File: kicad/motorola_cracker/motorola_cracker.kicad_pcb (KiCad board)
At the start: 2 copper layers, 115.1 x 46.5 mm, 28 parts, among them J1 DB9, P1 CONN_6, P2 CONN_2, P3 CONN_6, SW1 SWITCH_INV, U1 78L10, U2 74LS245, U3 MAX232, U4 78L05, U5 68HC05_PLCC, X1 4Mhz

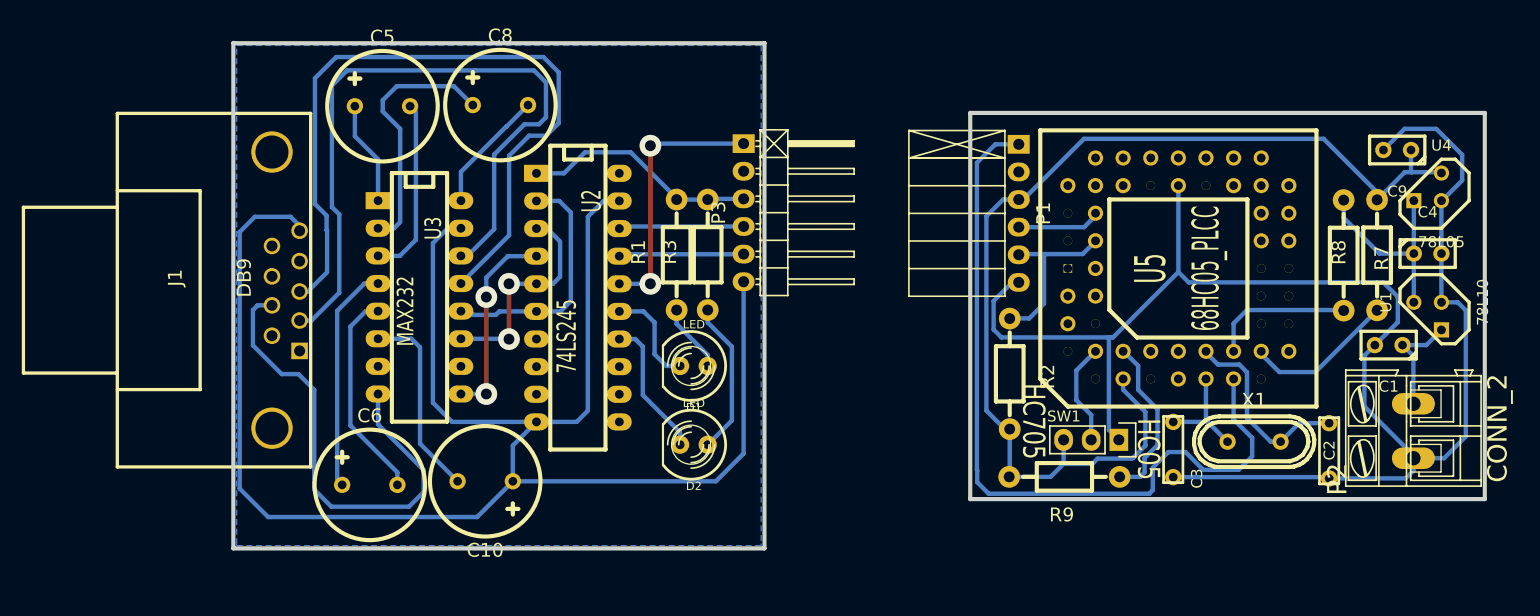
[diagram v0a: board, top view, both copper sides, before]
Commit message: motorola cracker simple board for usb to serial dongle (tested with cp2102)
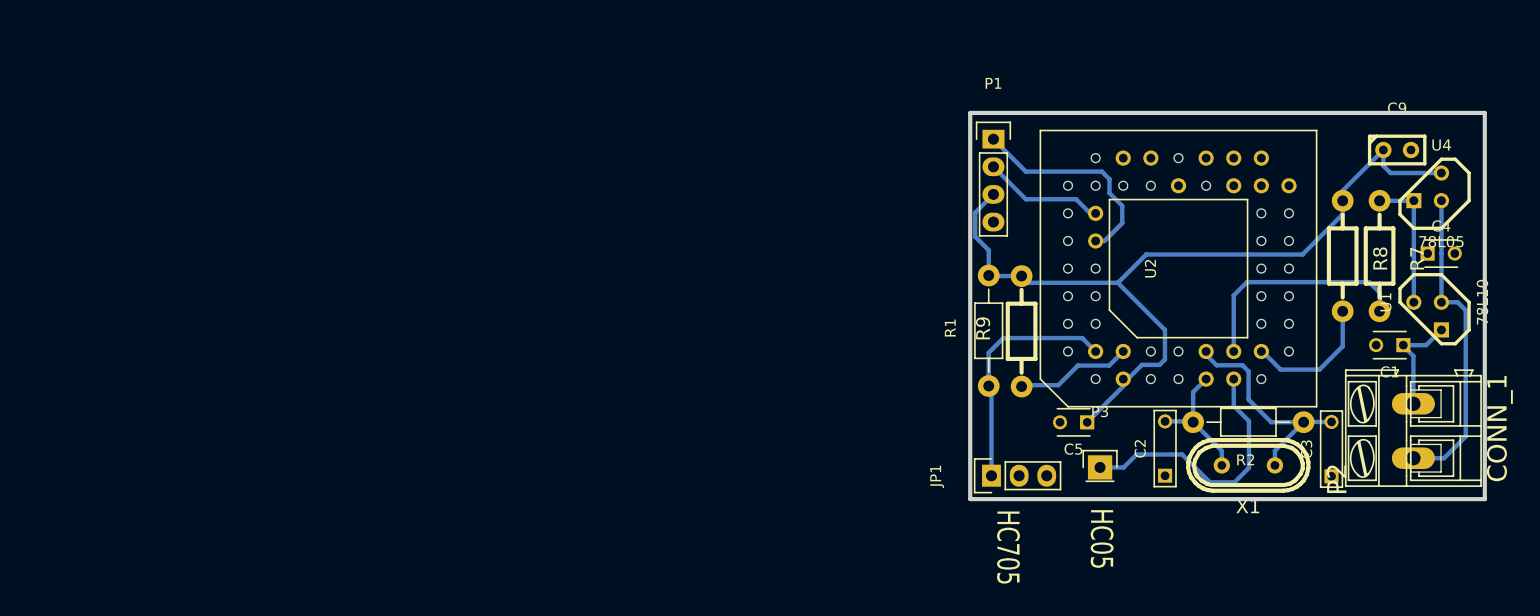
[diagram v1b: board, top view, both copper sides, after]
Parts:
- removed C10, C6, C8: 10m, Capacitors_Elko_ThroughHole:Elko_vert_DM10_RM5
- removed D1, D2: LED, LEDs:LED-5MM
- removed J1: DB9, Connect:DB9FC
- removed R3: 1k, Resistors_ThroughHole:Resistor_Horizontal_RM10mm
- removed SW1: SWITCH_INV, Pin_Headers:Pin_Header_Straight_1x03
- removed U3: MAX232, Sockets_DIP:DIP-16__300_ELL
- removed U5: 68HC05_PLCC, Sockets:PLCC52
- added JP1: JUMPER3, Pin_Headers:Pin_Header_Straight_1x03, F.Cu at (186.4, 117.9)
- C1, C4: footprint Capacitors_ThroughHole:Capacitor3MMDiscRM2.5 -> Capacitors_ThroughHole:C_Disc_D3_P2.5
- C2, C3: footprint Capacitors_ThroughHole:Capacitor6MMDiscRM5 -> Capacitors_ThroughHole:C_Rect_L7_W2_P5
- C5: value 10m -> 100n; footprint Capacitors_Elko_ThroughHole:Elko_vert_DM10_RM5 -> Capacitors_ThroughHole:C_Disc_D3_P2.5
- P1: value CONN_6 -> CONN_4; footprint Socket_Strips:Socket_Strip_Angled_1x06 -> Pin_Headers:Pin_Header_Straight_1x04
- P2: value CONN_2 -> CONN_1
- P3: value CONN_6 -> CONN_5; footprint Pin_Headers:Pin_Header_Angled_1x06 -> Pin_Headers:Pin_Header_Straight_1x01
- R1: value 1k -> 10k
- R2: value 4k7 -> 100M
- R8, R9: value 2k -> 1k
- U2: value 74LS245 -> 68HC05_PLCC; footprint Sockets_DIP:DIP-20__300_ELL -> Sockets:PLCC52
- moved C5 71.0 mm to (195.2, 112.9), turned to 180 degrees
- moved U2 55.3 mm to (203.6, 98.8), turned to 90 degrees
- moved P3 40.3 mm to (196.4, 117.1), turned to 0 degrees
- moved R1 29.5 mm to (186.2, 104.5)
- moved R2 22.4 mm to (210.1, 112.9), turned to 180 degrees
- moved C2 15.3 mm to (202.4, 117.9)
- moved C3 14.8 mm to (217.7, 117.9)
- moved R9 14.0 mm to (189.2, 104.6), turned to 90 degrees
- moved P1 7.21 mm to (186.6, 86.9), turned to 0 degrees
- moved R7 3.30 mm to (222.1, 97.7)
- moved R8 3.16 mm to (218.7, 97.7), turned to 270 degrees
- moved X1 2.24 mm to (210.1, 116.9), turned to 180 degrees
- moved C1 1.35 mm to (224.3, 105.8)
- turned C9 to 0 degrees
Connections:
- net +10V renamed /+10V
- C5 pad 1: Net-(C5-Pad1) -> +5V
- C5 pad 2: Net-(C5-Pad2) -> GND
- P1 pad 1: 68_18 -> /TX
- P1 pad 2: (no net) -> /RX
- P1 pad 4: 68_50 -> GND
- P3 pad 1: 68_18 -> /RESET
- R1 pad 1: Net-(D1-Pad1) -> Net-(JP1-Pad1)
- R2 pad 1: 68_52 -> Net-(C3-Pad2)
- R2 pad 2: +5V -> Net-(C2-Pad2)
- R8 pad 1: Net-(R8-Pad1) -> +5V
- R8 pad 2: +5V -> Net-(R8-Pad2)
- U2 pad 10: GND -> +5V
- U2 pad 11: (no net) -> Net-(R9-Pad1)
- U2 pad 14: Net-(D2-Pad2) -> (no net)
- U2 pad 15: Net-(D1-Pad2) -> (no net)
- U2 pad 16: 68_18 -> Net-(C2-Pad2)
- U2 pad 17: 68_52 -> Net-(C3-Pad2)
- U2 pad 18: 68_50 -> /RESET
- U2 pad 19: GND -> Net-(R7-Pad2)
- U2 pad 2: Rx -> (no net)
- U2 pad 3: Tx -> (no net)
- U2 pad 4: Reset -> (no net)
- U2 pad 5: Tx -> (no net)
- U2 pad 6: Rx -> (no net)
- U2 pad 9: (no net) -> Net-(JP1-Pad1)
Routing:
- net GND: track 306.8 -> 29.5 mm
- net 68_18: track 95.7 -> 0.00 mm, vias 2 -> 0
- net Net-(J1-Pad3): track 69.5 -> 0.00 mm
- net Net-(J1-Pad2): track 65.7 -> 0.00 mm
- net Net-(J1-Pad7): track 43.7 -> 0.00 mm
- net +5V: track 120.8 -> 78.1 mm
- net 68_52: track 27.7 -> 0.00 mm
- net /RESET: track 0.00 -> 24.5 mm
- net Net-(C8-Pad1): track 23.7 -> 0.00 mm
- net Rx: track 22.8 -> 0.00 mm
- net Net-(JP1-Pad1): track 0.00 -> 22.4 mm
- net Net-(C6-Pad1): track 21.8 -> 0.00 mm
- net Tx: track 20.5 -> 0.00 mm, vias 2 -> 0
- net Net-(C6-Pad2): track 20.4 -> 0.00 mm
- net /TX: track 0.00 -> 19.9 mm
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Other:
- board size 115.1 x 46.5 mm -> 47.3 x 35.5 mm

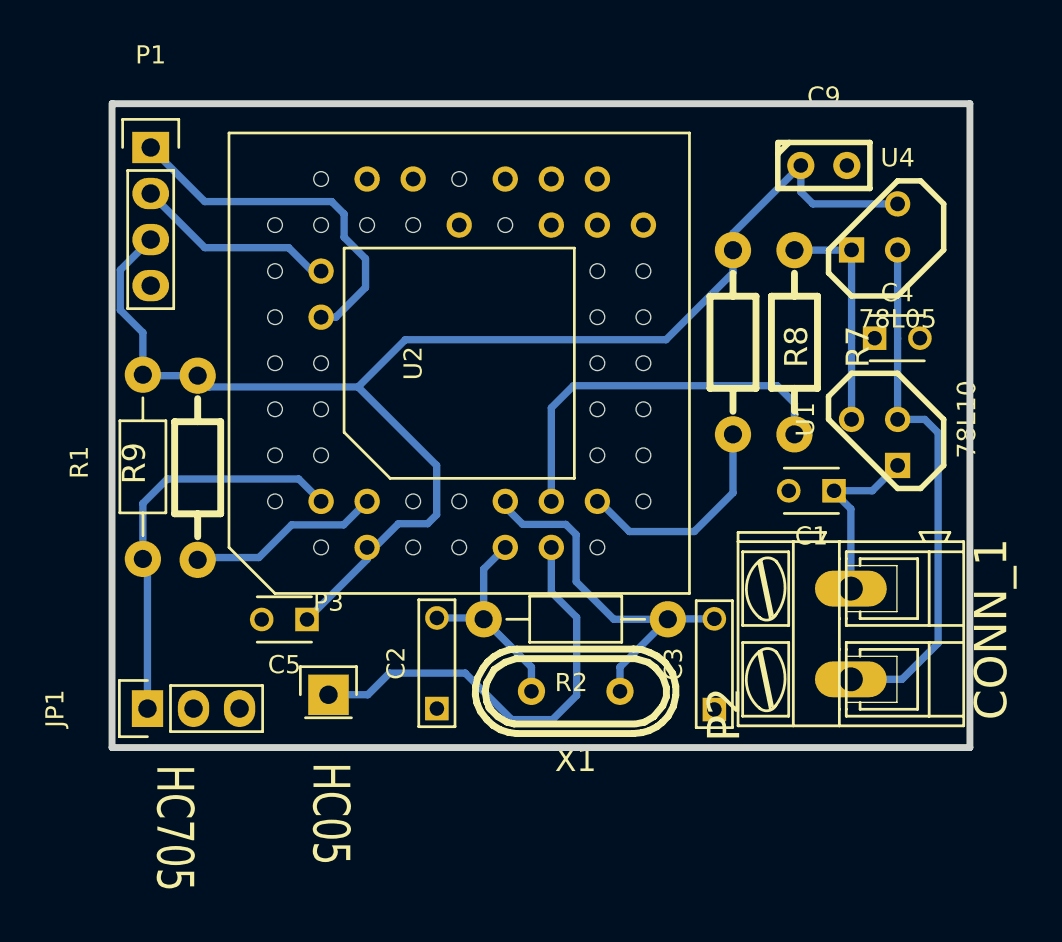
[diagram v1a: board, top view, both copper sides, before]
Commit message: simplified version
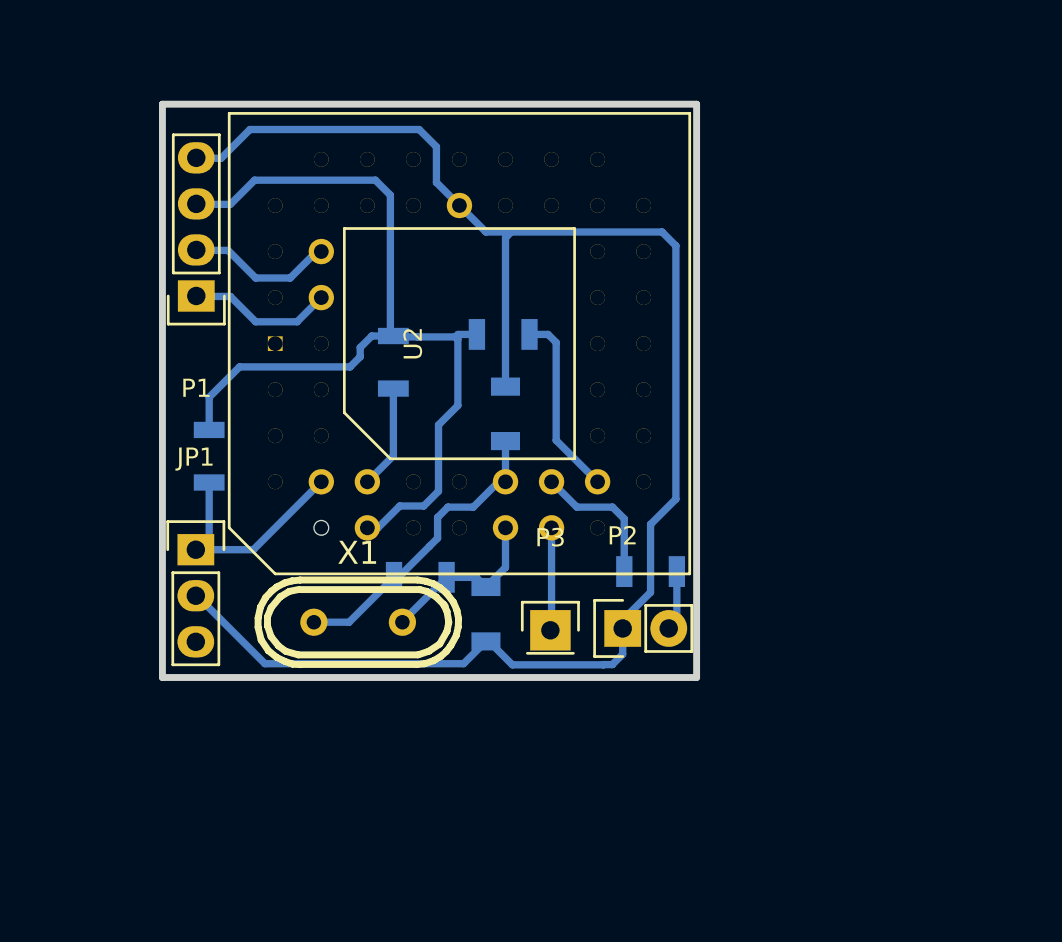
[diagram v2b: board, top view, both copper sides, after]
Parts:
- removed C1, C4, C5: 100n, Capacitors_ThroughHole:C_Disc_D3_P2.5
- removed C9: 100n, Capacitors_ThroughHole:Capacitor3MMDiscRM2.5
- removed U1: 78L10, my_modules:TO92-STABIL
- removed U4: 78L05, my_modules:TO92-STABIL
- C2, C3: footprint Capacitors_ThroughHole:C_Rect_L7_W2_P5 -> Capacitors_SMD:C_1206; moved to B.Cu
- P1: value CONN_4 -> UART
- P2: value CONN_1 -> +12V; footprint Connect:AK300-2 -> Socket_Strips:Socket_Strip_Straight_1x02
- P3: value CONN_5 -> RTS
- R1, R2, R7, R8, R9: footprint Resistors_ThroughHole:Resistor_Horizontal_RM10mm -> Resistors_SMD:R_1206; moved to B.Cu
- moved C3 20.0 mm to (206.2, 101.6), turned to 270 degrees
- moved R7 14.9 mm to (214.2, 110.3), turned to 180 degrees
- moved P3 12.7 mm to (208.7, 113.5)
- moved R8 12.7 mm to (206.1, 97.2), turned to 0 degrees
- moved X1 12.6 mm to (198.1, 113.1), turned to 0 degrees
- moved P2 12.6 mm to (212.6, 113.4), turned to 0 degrees
- moved R9 12.3 mm to (200.0, 98.8)
- moved JP1 9.16 mm to (189.1, 109.1), turned to 0 degrees
- moved R2 8.88 mm to (201.5, 110.6), turned to 0 degrees
- moved P1 8.57 mm to (189.1, 95.1), turned to 180 degrees
- moved C2 5.87 mm to (205.1, 112.6)
- moved R1 3.70 mm to (189.8, 103.9)
- moved U2 1.08 mm to (203.6, 97.7)
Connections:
- P2 pad 2: Net-(C1-Pad1) -> /+12V
- R7 pad 1: /+10V -> /+12V
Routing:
- net GND: track 29.5 -> 90.7 mm
- net +5V: track 78.1 -> 52.5 mm
- net /RESET: track 24.5 -> 5.91 mm
- net Net-(R7-Pad2): track 21.7 -> 7.96 mm
- net /+10V: track 12.5 -> 0.00 mm
- net /TX: track 19.9 -> 7.86 mm
- net Net-(C1-Pad1): track 9.97 -> 0.00 mm
- net Net-(JP1-Pad1): track 22.4 -> 12.5 mm
- net Net-(R9-Pad1): track 11.0 -> 5.76 mm
- net Net-(C3-Pad2): track 21.5 -> 17.4 mm
- net /+12V: track 0.00 -> 3.70 mm
- net /RX: track 11.6 -> 8.22 mm
- net Net-(R8-Pad2): track 12.7 -> 10.3 mm
- net Net-(C2-Pad2): track 12.1 -> 10.6 mm
- removed copper zone on B.Cu, net GND
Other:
- board size 47.3 x 35.5 mm -> 29.5 x 31.6 mm
- board text removed: "HC05"
- board text removed: "HC705"
